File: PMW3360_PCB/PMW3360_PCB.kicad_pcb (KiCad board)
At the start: 2 copper layers, 27 x 22.9 mm, 20 parts, among them J1 Conn_01x08, U1 PMW3360DM-T2QU, U2 TPS73601DBV

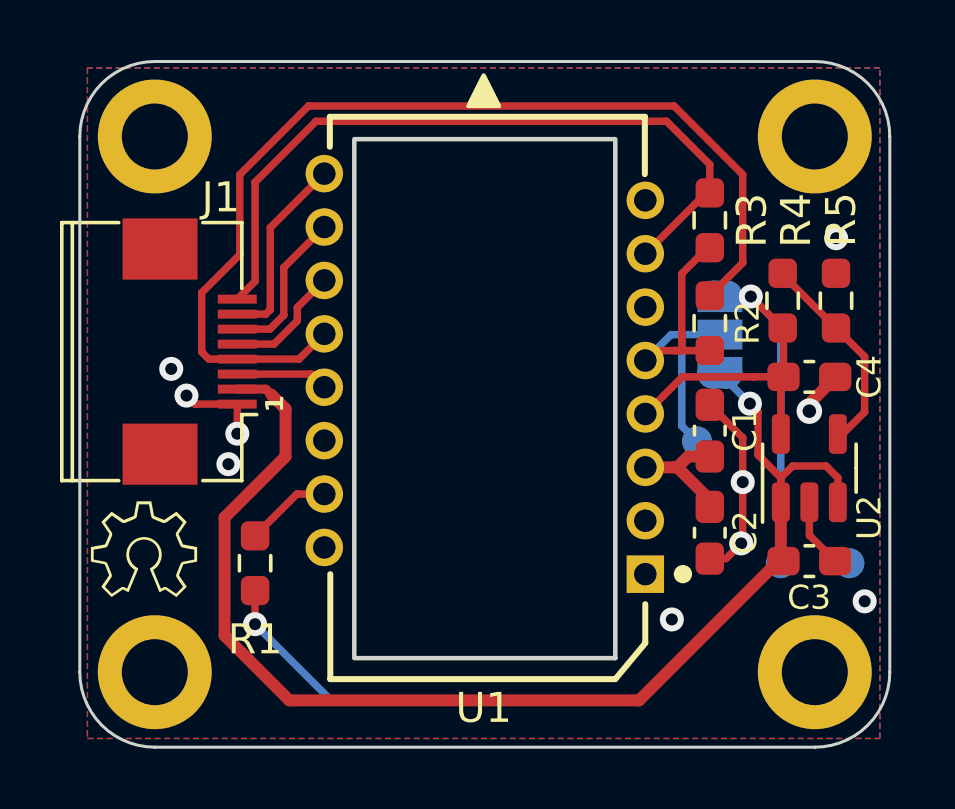
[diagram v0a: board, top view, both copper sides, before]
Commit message: Update schematic
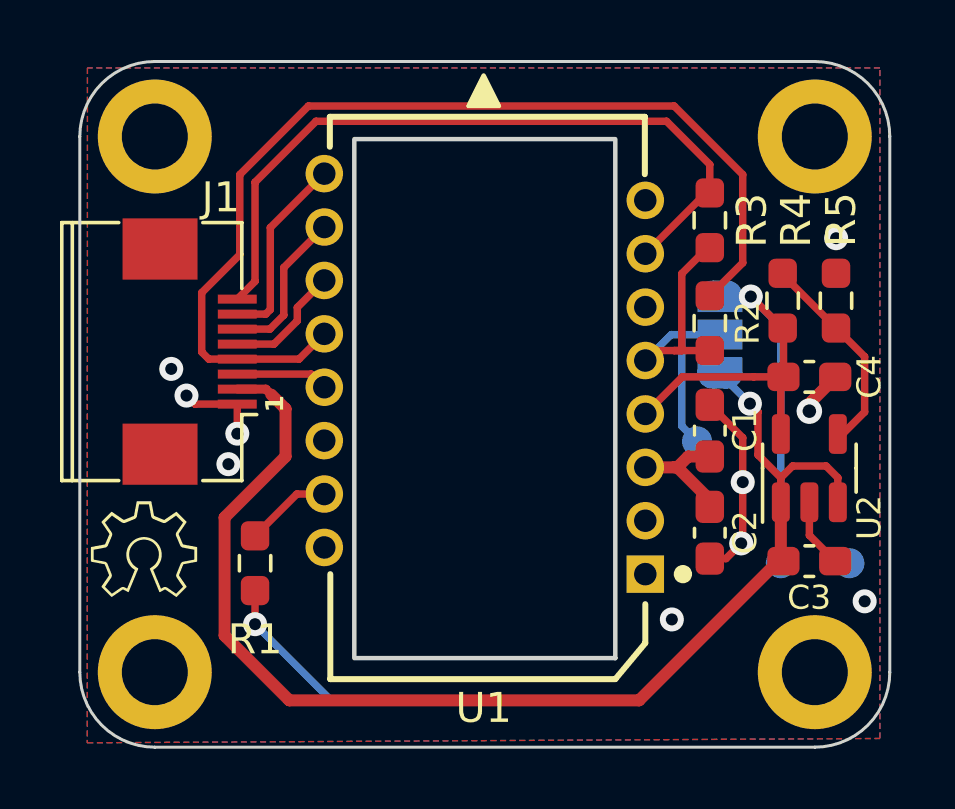
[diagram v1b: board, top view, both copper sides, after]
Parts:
- J1: value Conn_01x08 -> Interface
- TP1: value V_{IO} Test -> V_{IO}
- TP2: value V_{DD} Test -> V_{DD}
- TP3: value GND Test -> GND
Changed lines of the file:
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@@
     (title "PMW3360 PCB")
     (rev "3.2")
+    (company "SideraKB")
     (comment 1 "PMW3360DM-T2QU optical mouse sensor breakout board")
     (comment 2 "MIT License (Open Source Hardware)")
@@
         (effects (font (size 1 1) (thickness 0.15)))
     )
-    (fp_text value "Conn_01x08" (at 0 0.5 90 unlocked) (layer "F.Fab")
+    (fp_text value "Interface" (at 0 0.5 90 unlocked) (layer "F.Fab")
         (effects (font (size 1 1) (thickness 0.15)))
     )
@@
         (effects (font (size 1 1) (thickness 0.15)) (justify mirror))
     )
-    (fp_text value "V_{DD} Test" (at 0 -1.55) (layer "B.Fab")
+    (fp_text value "V_{DD}" (at 0 -1.55) (layer "B.Fab")
         (effects (font (size 1 1) (thickness 0.15)) (justify mirror))
     )
@@
         (effects (font (size 1 1) (thickness 0.15)) (justify mirror))
     )
-    (fp_text value "V_{IO} Test" (at 0 -1.55) (layer "B.Fab")
+    (fp_text value "V_{IO}" (at 0 -1.55) (layer "B.Fab")
         (effects (font (size 1 1) (thickness 0.15)) (justify mirror))
     )
@@
         (effects (font (size 1 1) (thickness 0.15)) (justify mirror))
     )
-    (fp_text value "GND Test" (at 0 -1.55) (layer "B.Fab")
+    (fp_text value "GND" (at 0 -1.55) (layer "B.Fab")
         (effects (font (size 1 1) (thickness 0.15)) (justify mirror))
     )
@@
   (segment (start 193.557 130.6418) (end 193.917 130.2818) (width 0.4) (layer "F.Cu") (net 1))
   (segment (start 193.917 130.2818) (end 194.639 130.2818) (width 0.4) (layer "F.Cu") (net 1))
-  (segment (start 195.1793 133.6843) (end 194.639 133.6843) (width 0.25) (layer "F.Cu") (net 2))
+  (segment (start 195.737 133.1266) (end 195.1793 133.6843) (width 0.25) (layer "F.Cu") (net 2))
   (segment (start 197.957 128.7688) (end 197.957 128.5148) (width 0.4) (layer "F.Cu") (net 2))
   (segment (start 197.957 132.9063) (end 198.8195 133.7688) (width 0.25) (layer "F.Cu") (net 2))
-  (segment (start 195.737 133.1266) (end 195.1793 133.6843) (width 0.25) (layer "F.Cu") (net 2))
-  (segment (start 195.737 129.6548) (end 195.737 133.1266) (width 0.25) (layer "F.Cu") (net 2))
   (segment (start 177.479 128.5338) (end 177.195 128.2498) (width 0.25) (layer "F.Cu") (net 2))
   (segment (start 178.889 128.5338) (end 178.889 129.5198) (width 0.25) (layer "F.Cu") (net 2))
-  (segment (start 194.639 128.5568) (end 195.737 129.6548) (width 0.25) (layer "F.Cu") (net 2))
+  (segment (start 195.737 129.6548) (end 195.737 133.1266) (width 0.25) (layer "F.Cu") (net 2))
   (segment (start 198.8195 127.6523) (end 198.8195 127.6258) (width 0.25) (layer "F.Cu") (net 2))
   (segment (start 178.889 128.5338) (end 177.479 128.5338) (width 0.25) (layer "F.Cu") (net 2))
+  (segment (start 195.1793 133.6843) (end 194.639 133.6843) (width 0.25) (layer "F.Cu") (net 2))
   (segment (start 197.957 128.5148) (end 198.8195 127.6523) (width 0.4) (layer "F.Cu") (net 2))
+  (segment (start 194.639 128.5568) (end 195.737 129.6548) (width 0.25) (layer "F.Cu") (net 2))
   (segment (start 197.957 131.8058) (end 197.957 132.9063) (width 0.25) (layer "F.Cu") (net 2))
   (via (at 193.374106 135.71235) (size 0.8) (drill 0.4) (layers "F.Cu" "B.Cu") (free) (net 2))
@@
   (segment (start 197.068 124.1733) (end 197.068 124.2203) (width 0.25) (layer "F.Cu") (net 13))
   (zone (net 2) (net_name "GND") (layers "F&B.Cu") (hatch edge 0.508)
-    (connect_pads (clearance 0.508))
+    (connect_pads (clearance 0.5))
     (min_thickness 0.254) (filled_areas_thickness no)
     (fill yes (thermal_gap 0.508) (thermal_bridge_width 0.508))
     (polygon
       (pts
-        (xy 173.893 139.6798)
+        (xy 173.889 139.8238)
         (xy 200.309 139.6798)
         (xy 200.309 117.3278)

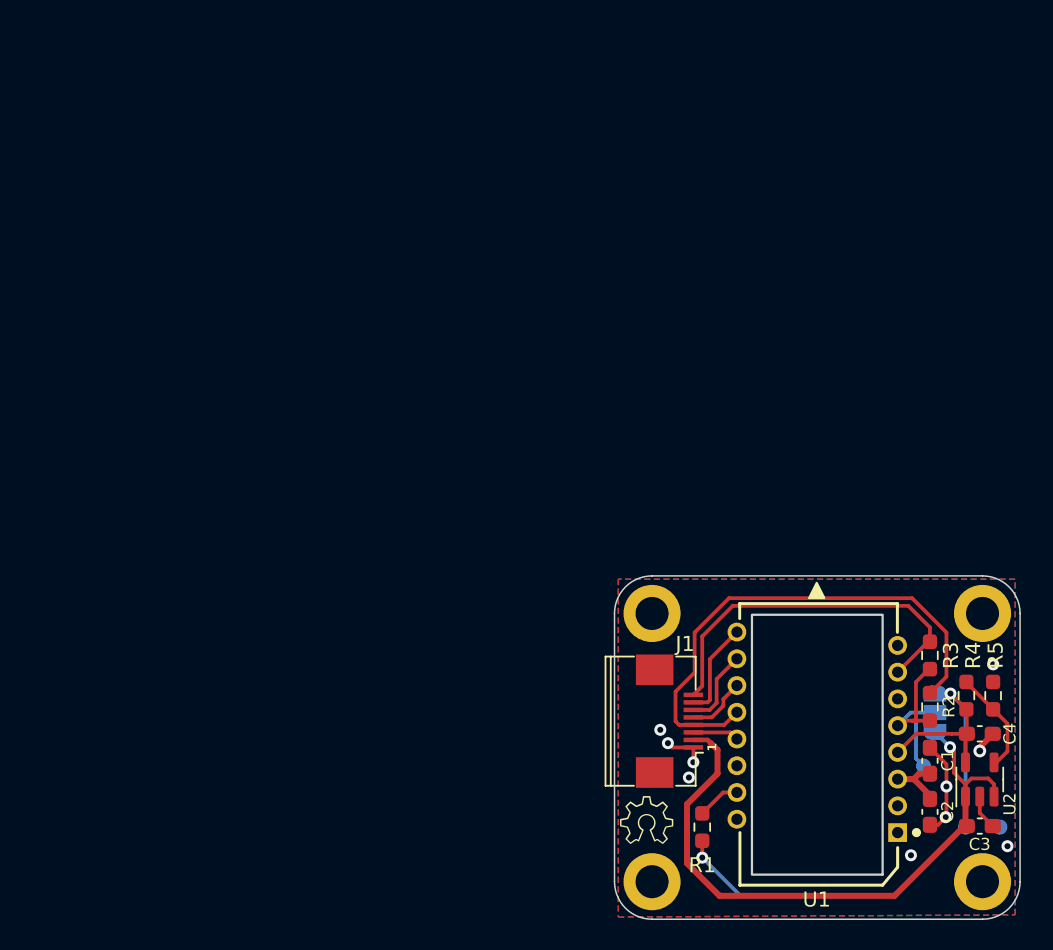
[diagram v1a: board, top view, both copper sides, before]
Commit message: Rerounted
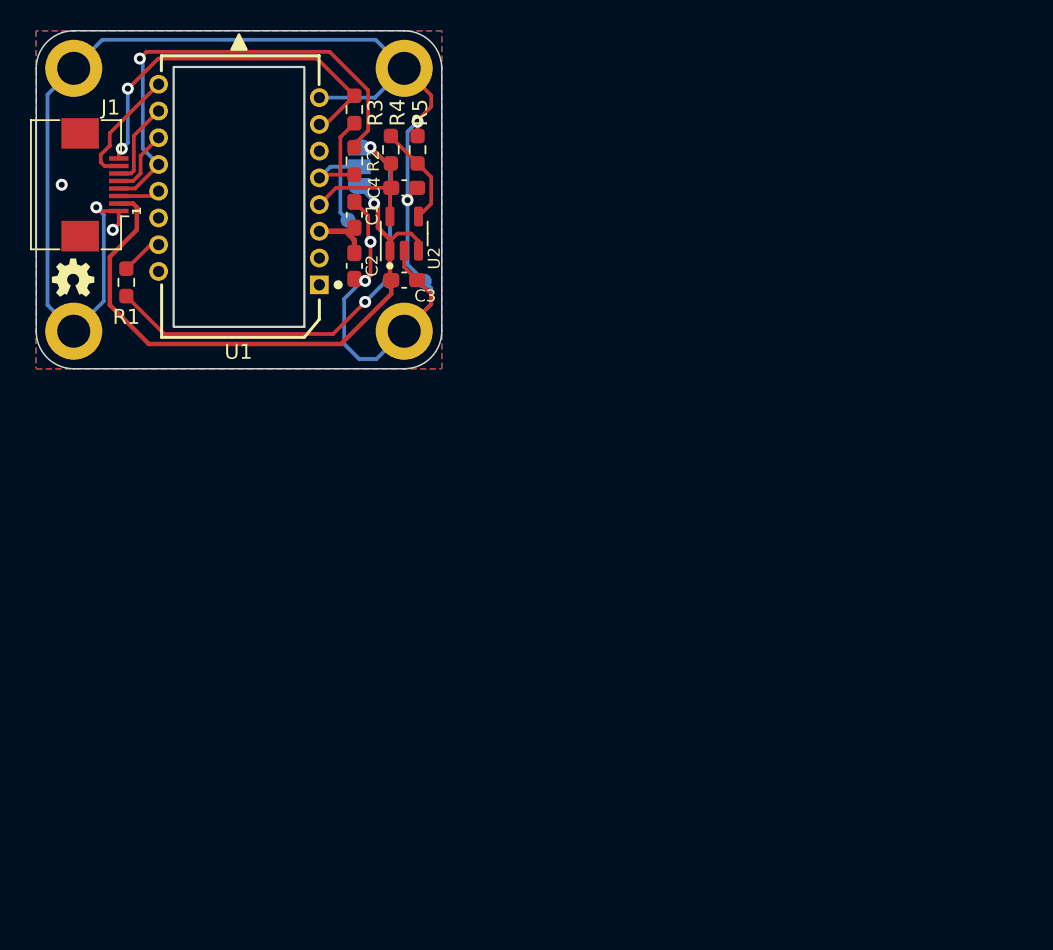
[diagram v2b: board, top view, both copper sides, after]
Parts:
- moved H1 53.2 mm to (137.6, 100.8)
- moved H2 53.2 mm to (159.6, 100.8)
- moved U1 53.0 mm to (148.6, 91.6)
- moved H3 52.9 mm to (159.6, 83.3)
- moved H4 52.9 mm to (137.6, 83.3)
- moved R4 52.8 mm to (158.8, 88.7)
- moved R5 52.8 mm to (160.5, 88.7)
- moved C1 52.8 mm to (156.3, 93.1)
- moved C2 52.8 mm to (156.3, 96.5)
- moved R2 52.8 mm to (156.3, 89.5)
- moved R3 52.8 mm to (156.3, 86.1)
- moved TP2 52.8 mm to (158.7, 97.5)
- moved TP3 52.8 mm to (161.0, 97.5)
- moved C3 52.8 mm to (159.6, 97.4)
- moved C4 52.8 mm to (159.6, 91.3)
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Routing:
- net GND: track 13.0 -> 107.2 mm, vias 10 -> 7
- net /MISO: track 34.1 -> 31.5 mm, vias 0 -> 1
- net Net-(U1-VDDPIX): track 4.06 -> 5.86 mm
- net /MOTION: track 6.44 -> 8.09 mm
- net VDD: track 42.1 -> 40.9 mm
- net V_{IN}: track 41.9 -> 41.4 mm
- net /RESET: track 24.7 -> 25.0 mm, vias 0 -> 2
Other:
- board size 27 x 22.9 mm -> 27 x 22.5 mm
- board text added: "2"
